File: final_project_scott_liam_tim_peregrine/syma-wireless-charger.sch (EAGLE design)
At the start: 46 parts, among them U1 SAMD21E

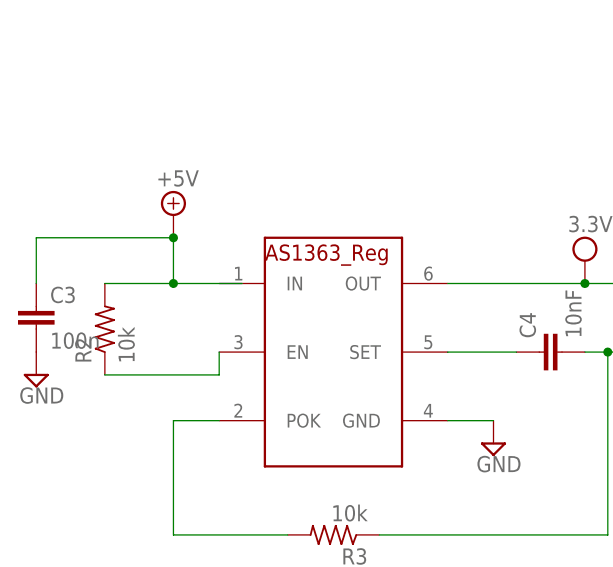
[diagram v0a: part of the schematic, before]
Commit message: Fixed errors
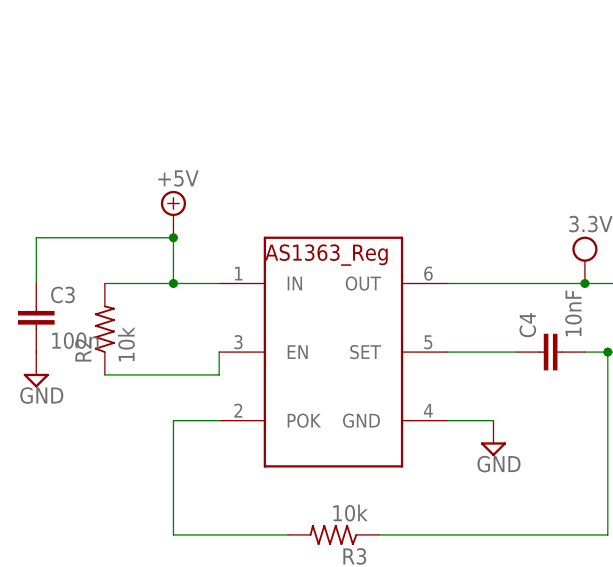
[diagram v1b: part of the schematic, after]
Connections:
- removed net 3.3V: U$6.VDD
- net +5V: now also U2.IN
- net VDD: now also U$6.VDD
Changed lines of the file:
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@@
 <?xml version="1.0" encoding="utf-8"?>
 <!DOCTYPE eagle SYSTEM "eagle.dtd">
-<eagle version="7.4.0">
+<eagle version="7.5.0">
 <drawing>
 <settings>
@@
 <part name="SUPPLY29" library="supply2" deviceset="GND" device=""/>
 <part name="SUPPLY30" library="supply2" deviceset="VDD" device="" value="3.3V"/>
-<part name="SUPPLY31" library="supply2" deviceset="VDD" device="" value="3.3V"/>
 <part name="C14" library="rcl" deviceset="C-EU" device="C1206" value="100n"/>
 <part name="U$8" library="foe-scale" deviceset="SCHTKYDIODE-523" device=""/>
@@
 <part name="U$9" library="foe-scale" deviceset="LTST-C193KGKT_GREEN-LED" device=""/>
 <part name="C15" library="resistor" deviceset="C-EU" device="C0603" value="100n"/>
+<part name="SUPPLY31" library="supply2" deviceset="VDD" device="" value="3.3V"/>
 </parts>
 <sheets>
@@
 <instance part="SUPPLY29" gate="GND" x="121.92" y="-12.7"/>
 <instance part="SUPPLY30" gate="G$1" x="175.26" y="-2.54"/>
-<instance part="SUPPLY31" gate="G$1" x="172.72" y="50.8"/>
 <instance part="C14" gate="G$1" x="78.74" y="58.42" rot="R270"/>
 <instance part="U$8" gate="G$1" x="60.96" y="15.24"/>
@@
 <instance part="U$9" gate="G$1" x="7.62" y="78.74"/>
 <instance part="C15" gate="G$1" x="91.44" y="35.56"/>
+<instance part="SUPPLY31" gate="G$1" x="172.72" y="50.8"/>
 </instances>
 <busses>
@@
 <wire x1="-106.68" y1="22.86" x2="-106.68" y2="27.94" width="0.1524" layer="91"/>
 <pinref part="R2" gate="G$1" pin="2"/>
-<wire x1="-83.82" y1="22.86" x2="-91.44" y2="22.86" width="0.1524" layer="91"/>
 <wire x1="-91.44" y1="22.86" x2="-99.06" y2="22.86" width="0.1524" layer="91"/>
 <wire x1="-106.68" y1="27.94" x2="-91.44" y2="27.94" width="0.1524" layer="91"/>
 <wire x1="-91.44" y1="27.94" x2="-91.44" y2="22.86" width="0.1524" layer="91"/>
-<junction x="-91.44" y="22.86"/>
 <pinref part="SUPPLY4" gate="+5V" pin="+5V"/>
 <junction x="-91.44" y="27.94"/>
+<pinref part="U2" gate="AS1363" pin="IN"/>
+<wire x1="-91.44" y1="22.86" x2="-86.36" y2="22.86" width="0.1524" layer="91"/>
+<junction x="-91.44" y="22.86"/>
 </segment>
 <segment>
@@
 </segment>
 <segment>
-<pinref part="U$7" gate="G$1" pin="VDD"/>
-<wire x1="152.4" y1="48.26" x2="172.72" y2="48.26" width="0.1524" layer="91"/>
-<pinref part="SUPPLY31" gate="G$1" pin="VDD"/>
-</segment>
-<segment>
 <pinref part="R15" gate="G$1" pin="2"/>
 <wire x1="208.28" y1="-17.78" x2="208.28" y2="-12.7" width="0.1524" layer="91"/>
 <pinref part="SUPPLY35" gate="G$1" pin="VDD"/>
+</segment>
+<segment>
+<pinref part="U$7" gate="G$1" pin="VDD"/>
+<pinref part="SUPPLY31" gate="G$1" pin="VDD"/>
+<wire x1="152.4" y1="48.26" x2="172.72" y2="48.26" width="0.1524" layer="91"/>
+</segment>
+<segment>
+<pinref part="U$6" gate="G$1" pin="VDD"/>
+<pinref part="SUPPLY30" gate="G$1" pin="VDD"/>
+<wire x1="152.4" y1="-5.08" x2="175.26" y2="-5.08" width="0.1524" layer="91"/>
 </segment>
 </net>
@@
 </segment>
 </net>
-<net name="3.3V" class="0">
-<segment>
-<pinref part="U$6" gate="G$1" pin="VDD"/>
-<wire x1="152.4" y1="-5.08" x2="175.26" y2="-5.08" width="0.1524" layer="91"/>
-<pinref part="SUPPLY30" gate="G$1" pin="VDD"/>
-</segment>
-</net>

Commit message: fixed errors, added aesthetic silkscreen
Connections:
- removed net N$8: C1.2, R6.1, U$1.IMON
- net IMON: now also C1.2, R6.1, U$1.IMON
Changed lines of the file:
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@@
-</segment>
-</net>
-<net name="N$8" class="0">
-<segment>
-<pinref part="R6" gate="G$1" pin="1"/>
-<pinref part="U$1" gate="G$1" pin="IMON"/>
-<wire x1="30.48" y1="91.44" x2="30.48" y2="81.28" width="0.1524" layer="91"/>
-<pinref part="C1" gate="G$1" pin="2"/>
-<wire x1="20.32" y1="93.98" x2="20.32" y2="91.44" width="0.1524" layer="91"/>
-<wire x1="20.32" y1="91.44" x2="30.48" y2="91.44" width="0.1524" layer="91"/>
-<junction x="30.48" y="91.44"/>
 </segment>
 </net>
@@
 <label x="-7.62" y="-53.34" size="1.778" layer="95"/>
 </segment>
+<segment>
+<pinref part="R6" gate="G$1" pin="1"/>
+<pinref part="U$1" gate="G$1" pin="IMON"/>
+<wire x1="30.48" y1="91.44" x2="30.48" y2="81.28" width="0.1524" layer="91"/>
+<pinref part="C1" gate="G$1" pin="2"/>
+<wire x1="20.32" y1="93.98" x2="20.32" y2="91.44" width="0.1524" layer="91"/>
+<wire x1="20.32" y1="91.44" x2="30.48" y2="91.44" width="0.1524" layer="91"/>
+<junction x="30.48" y="91.44"/>
+</segment>
 </net>
